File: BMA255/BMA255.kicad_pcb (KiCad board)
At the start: 2 copper layers, 25.4 x 17.8 mm, 26 parts, among them J1 Conn_01x06, J2 Conn_01x04, J3 Conn_01x06, J4 Conn_01x04, Q1 BSS138DW, Q2 BSS138DW, U1 AP2127K-3.3

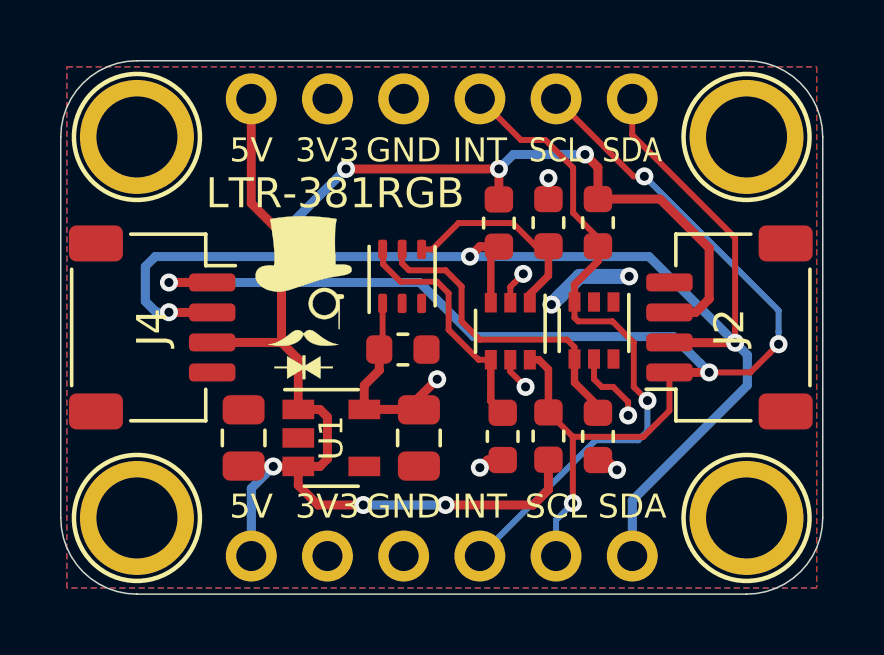
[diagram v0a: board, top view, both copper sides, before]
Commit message: Phew...
almost a screw up
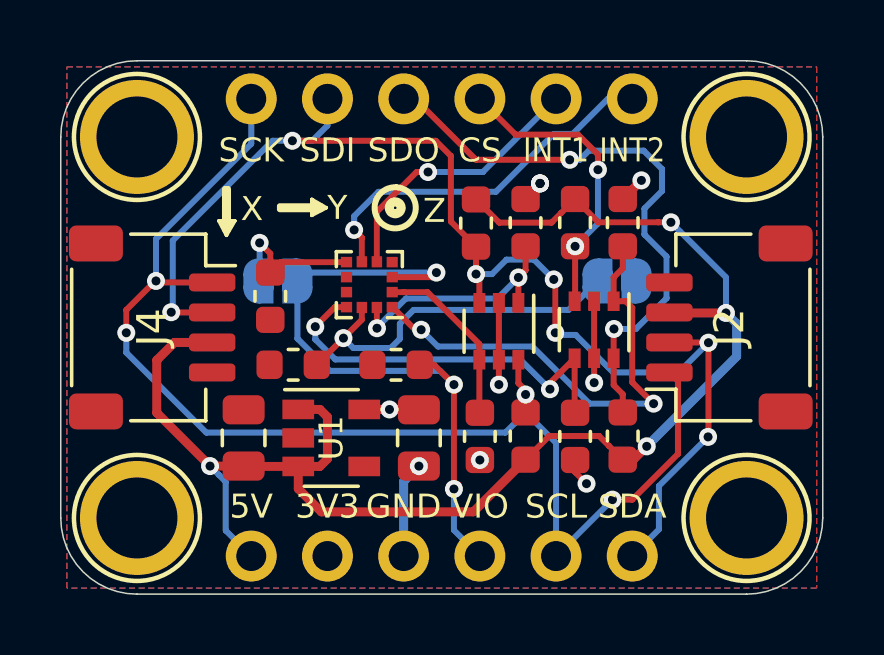
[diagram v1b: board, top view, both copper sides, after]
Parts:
- removed C2: 100nF, Capacitor_SMD:C_0603_1608Metric
- removed the G*** at (60.7, 35.0)
- removed LTR-381RGB: LTR-381RGB-WA, OptoDevice:Lite-On_LTR-303ALS-01
- added C3: 1uF, Capacitor_SMD:C_0603_1608Metric, F.Cu at (59.6, 34.9)
- added C5: 100nF, Capacitor_SMD:C_0603_1608Metric, F.Cu at (63.8, 37.2)
- added JP1: SolderJumper_2_Open, Jumper:SolderJumper-2_P1.3mm_Open_RoundedPad1.0x1.5mm, B.Cu at (59.8, 34.4)
- added JP2: SolderJumper_2_Open, Jumper:SolderJumper-2_P1.3mm_Open_RoundedPad1.0x1.5mm, B.Cu at (71.1, 34.4)
- added R1: 10K, Resistor_SMD:R_0603_1608Metric, F.Cu at (71.3, 32.5)
- added R2: 10K, Resistor_SMD:R_0603_1608Metric, F.Cu at (71.3, 39.6)
- added R9: 10K, Resistor_SMD:R_0603_1608Metric, F.Cu at (60.3, 37.2)
- added U2: BMA255, Package_LGA:LGA-12_2x2mm_P0.5mm, F.Cu at (62.9, 34.5)
- moved R3 0.76 mm to (69.7, 39.6)
- moved R4 0.76 mm to (69.7, 32.5)
- moved R5 0.76 mm to (68.1, 32.5)
- moved R6 0.76 mm to (68.1, 39.6)
- moved R7 0.76 mm to (66.5, 39.6)
- moved R8 0.76 mm to (66.4, 32.5)
- moved Q2 0.38 mm to (67.2, 36.1)
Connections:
- net INT_3V3 renamed CS_3V3
- J1 pad 4: INT_5V -> VDDIO
- J3 pad 1: 5V -> SCL_5V
- J3 pad 2: 3V3 -> SDA_5V
- J3 pad 3: GND -> SDO_5V
- J3 pad 4: INT_5V -> CS_5V
- J3 pad 5: SCL_5V -> INT1
- J3 pad 6: SDA_5V -> INT2
- Q1 pad 1: (no net) -> SDO_3V3
- Q1 pad 2: (no net) -> 3V3
- Q1 pad 3: INT_5V -> CS_5V
- Q1 pad 6: (no net) -> SDO_5V
- R4 pad 2: INT_5V -> CS_5V
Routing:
- net INT_5V: track 22.5 -> 0.00 mm, vias 1 -> 0
- net VDDIO: track 0.00 -> 21.8 mm, vias 0 -> 3
- net SDO_5V: track 0.00 -> 19.8 mm, vias 0 -> 2
- net SDO_3V3: track 0.00 -> 16.2 mm, vias 0 -> 2
- net INT2: track 0.00 -> 12.5 mm, vias 0 -> 1
- net Net-(JP2-Pad1): track 0.00 -> 12.4 mm, vias 0 -> 1
- net CS_5V: track 0.00 -> 9.92 mm, vias 0 -> 2
- net INT1: track 0.00 -> 9.20 mm, vias 0 -> 1
- net SCL_5V: track 48.6 -> 42.7 mm, vias 5 -> 4
- net SDA_5V: track 48.2 -> 42.6 mm, vias 3 -> 7
- net 5V: track 53.9 -> 49.6 mm, vias 7 -> 4
- net CS_3V3: track 10.6 -> 13.5 mm, vias 0 -> 2
- net SDA_3V3: track 8.07 -> 6.15 mm
- net 3V3: track 14.1 -> 15.3 mm, vias 7 -> 9
- net SCL_3V3: track 7.05 -> 8.10 mm, vias 0 -> 2
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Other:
- board text added: "12 Bit Acc."
- board text added: "BMA255 3 DOF Sensor"
- board text added: "CS"
- board text added: "Close for VDD=VDDIO"
- board text added: "Closed=I2C Open = SPI"
- board text added: "INT1"
- board text added: "INT2"
- board text added: "SCK"
- board text added: "SDI"
- board text added: "SDO"
- board text added: "VIO"
- board text added: "X"
- board text added: "Y"
- board text added: "Z"
- board text added: "±2g, ±4g, ±8g, ±16g"
- board text removed: "Address: Write-0xA6 Read-0xA7"
- board text removed: "Ambient Colour Infra-Red"
- board text removed: "INT"
- board text removed: "LTR-381RGB Sensor"

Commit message: Soldermask width adjusted
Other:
- rule solder_mask_min_width: 0.1 -> 0.05
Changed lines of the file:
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@@
   (layers
     (0 F.Cu signal)
-    (31 B.Cu signal hide)
+    (31 B.Cu signal)
     (32 B.Adhes user hide)
     (33 F.Adhes user hide)
@@
   )
   (setup
-    (last_trace_width 0.2)
+    (last_trace_width 0.127)
     (user_trace_width 0.2)
     (user_trace_width 0.25)
@@
     (pad_drill 1)
     (pad_to_mask_clearance 0)
-    (solder_mask_min_width 0.1)
+    (solder_mask_min_width 0.05)
     (aux_axis_origin 0 0)
     (visible_elements 7FFFFFFF)
